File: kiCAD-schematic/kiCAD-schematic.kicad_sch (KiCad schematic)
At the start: 39 parts, among them J1 ext. power, J2 keyboard (usb-a), J3 keyboard (ps/2), Q1 2N222A, Q2 2N3904, Q3 2N3906, Q4 2N3904, SW1 ~RESET, SW2 POWER

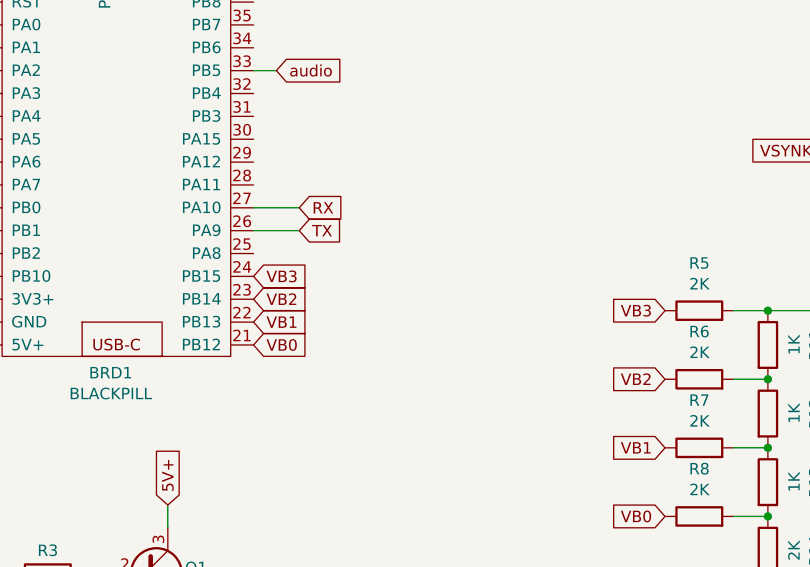
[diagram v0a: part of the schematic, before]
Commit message: modification de IF-SENSE
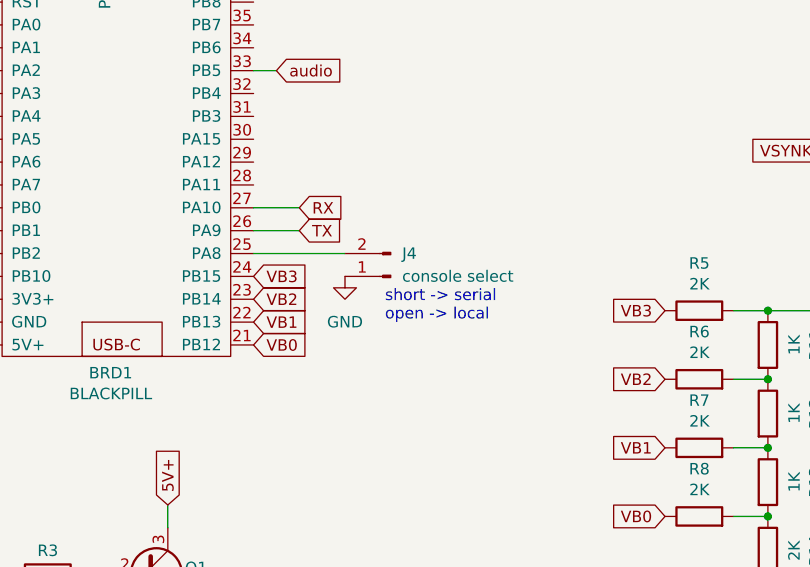
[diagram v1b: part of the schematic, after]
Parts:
- added J4: console select, symbol Connector:Conn_01x02_Male
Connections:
- net GND: now also J4.1 (Pin_1)
- net at BRD1.25 (PA8): now also J4.2 (Pin_2)
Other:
- note added: "short -> serial open -> local"
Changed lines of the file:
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@@
+    (stroke (width 0) (type default) (color 0 0 0 0))
+  )
+  (wire (pts (xy 163.83 110.49) (xy 173.99 110.49))
     (stroke (width 0) (type default) (color 0 0 0 0))
   )
@@
   (wire (pts (xy 210.82 16.51) (xy 214.63 16.51))
     (stroke (width 0) (type default) (color 0 0 0 0))
+  )
+  (text "short -> serial\nopen -> local" (at 178.435 118.11 0)
+    (effects (font (size 1.27 1.27)) (justify left bottom))
   )
   (text "keyboard connector\nalternative\n" (at 55.88 175.26 0)
@@
   (symbol (lib_id "power:GND") (at 214.63 35.56 0) (mirror y) (unit 1)
     (in_bom yes) (on_board yes)
-    (property "Reference" "#PWR011" (id 0) (at 214.63 41.91 0)
+    (property "Reference" "#PWR012" (id 0) (at 214.63 41.91 0)
       (effects (font (size 1.27 1.27)) hide)
     )
@@
   (symbol (lib_id "power:GND") (at 238.76 48.26 0) (unit 1)
     (in_bom yes) (on_board yes)
-    (property "Reference" "#PWR014" (id 0) (at 238.76 54.61 0)
+    (property "Reference" "#PWR015" (id 0) (at 238.76 54.61 0)
       (effects (font (size 1.27 1.27)) hide)
     )
@@
   (symbol (lib_id "power:GND") (at 248.92 133.35 0) (unit 1)
     (in_bom yes) (on_board yes)
-    (property "Reference" "#PWR015" (id 0) (at 248.92 139.7 0)
+    (property "Reference" "#PWR016" (id 0) (at 248.92 139.7 0)
       (effects (font (size 1.27 1.27)) hide)
     )
@@
   (symbol (lib_id "power:GND") (at 175.26 76.2 0) (unit 1)
     (in_bom yes) (on_board yes)
-    (property "Reference" "#PWR010" (id 0) (at 175.26 82.55 0)
+    (property "Reference" "#PWR011" (id 0) (at 175.26 82.55 0)
       (effects (font (size 1.27 1.27)) hide)
     )
@@
   (symbol (lib_id "power:GND") (at 234.95 133.35 0) (unit 1)
     (in_bom yes) (on_board yes)
-    (property "Reference" "#PWR013" (id 0) (at 234.95 139.7 0)
+    (property "Reference" "#PWR014" (id 0) (at 234.95 139.7 0)
       (effects (font (size 1.27 1.27)) hide)
     )
@@
   (symbol (lib_id "power:GND") (at 220.98 147.32 0) (unit 1)
     (in_bom yes) (on_board yes)
-    (property "Reference" "#PWR012" (id 0) (at 220.98 153.67 0)
+    (property "Reference" "#PWR013" (id 0) (at 220.98 153.67 0)
       (effects (font (size 1.27 1.27)) hide)
     )
@@
     (pin "2")
     (pin "3")
+  )
+  (symbol (lib_id "power:GND") (at 173.99 113.03 0) (unit 1)
+    (in_bom yes) (on_board yes) (fields_autoplaced)
+    (property "Reference" "#PWR010" (id 0) (at 173.99 119.38 0)
+      (effects (font (size 1.27 1.27)) hide)
+    )
+    (property "Value" "GND" (id 1) (at 173.99 118.11 0))
+    (property "Footprint" "" (id 2) (at 173.99 113.03 0)
+      (effects (font (size 1.27 1.27)) hide)
+    )
+    (property "Datasheet" "" (id 3) (at 173.99 113.03 0)
+      (effects (font (size 1.27 1.27)) hide)
+    )
+    (pin "1")
   )
   (symbol (lib_id "power:GND") (at 172.085 156.21 0) (unit 1)
@@
     (pin "2")
   )
+  (symbol (lib_id "Connector:Conn_01x02_Male") (at 179.07 113.03 180) (unit 1)
+    (in_bom yes) (on_board yes) (fields_autoplaced)
+    (property "Reference" "J4" (id 0) (at 180.34 110.4899 0)
+      (effects (font (size 1.27 1.27)) (justify right))
+    )
+    (property "Value" "console select" (id 1) (at 180.34 113.0299 0)
+      (effects (font (size 1.27 1.27)) (justify right))
+    )
+    (property "Footprint" "" (id 2) (at 179.07 113.03 0)
+      (effects (font (size 1.27 1.27)) hide)
+    )
+    (property "Datasheet" "~" (id 3) (at 179.07 113.03 0)
+      (effects (font (size 1.27 1.27)) hide)
+    )
+    (pin "1")
+    (pin "2")
+  )
   (sheet_instances
     (path "/" (page "1"))
@@
       (reference "#PWR09") (unit 1) (value "GND") (footprint "")
     )
+    (path "/293694f5-f84a-43cb-b18d-6048fb0e7311"
+      (reference "#PWR010") (unit 1) (value "GND") (footprint "")
+    )
     (path "/00000000-0000-0000-0000-00006002e243"
-      (reference "#PWR010") (unit 1) (value "GND") (footprint "")
+      (reference "#PWR011") (unit 1) (value "GND") (footprint "")
     )
     (path "/00000000-0000-0000-0000-00005ffbb8c6"
-      (reference "#PWR011") (unit 1) (value "GND") (footprint "")
+      (reference "#PWR012") (unit 1) (value "GND") (footprint "")
     )
     (path "/00000000-0000-0000-0000-0000606c01f2"
-      (reference "#PWR012") (unit 1) (value "GND") (footprint "")
+      (reference "#PWR013") (unit 1) (value "GND") (footprint "")
     )
     (path "/00000000-0000-0000-0000-0000606bce93"
-      (reference "#PWR013") (unit 1) (value "GND") (footprint "")
+      (reference "#PWR014") (unit 1) (value "GND") (footprint "")
     )
     (path "/00000000-0000-0000-0000-00005ffbd895"
-      (reference "#PWR014") (unit 1) (value "GND") (footprint "")
+      (reference "#PWR015") (unit 1) (value "GND") (footprint "")
     )
     (path "/00000000-0000-0000-0000-00005ffe2066"
-      (reference "#PWR015") (unit 1) (value "GND") (footprint "")
+      (reference "#PWR016") (unit 1) (value "GND") (footprint "")
     )
     (path "/00000000-0000-0000-0000-00005ffb52d6"
@@
       (reference "J3") (unit 1) (value "keyboard (ps/2)") (footprint "")
     )
+    (path "/e378ab9b-373b-45f1-b4f3-44620429fe99"
+      (reference "J4") (unit 1) (value "console select") (footprint "")
+    )
     (path "/a7b6ec0b-19e1-478b-92f2-5a0b45d45460"

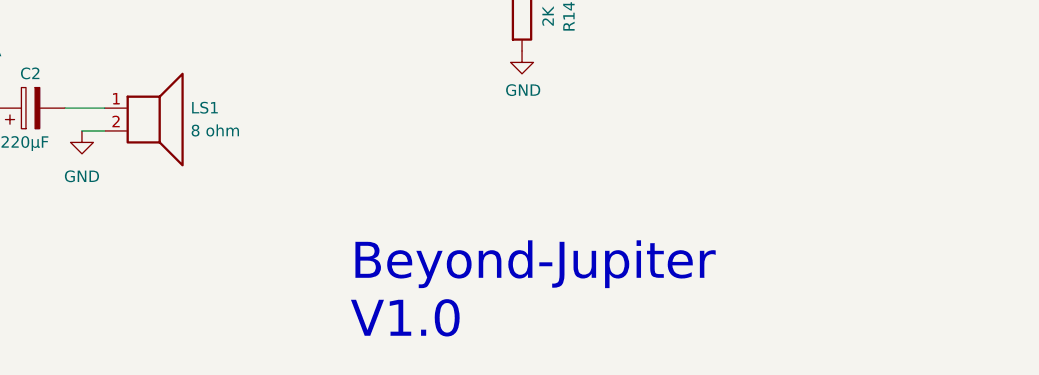
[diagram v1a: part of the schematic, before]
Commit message: mise à jour readme.md
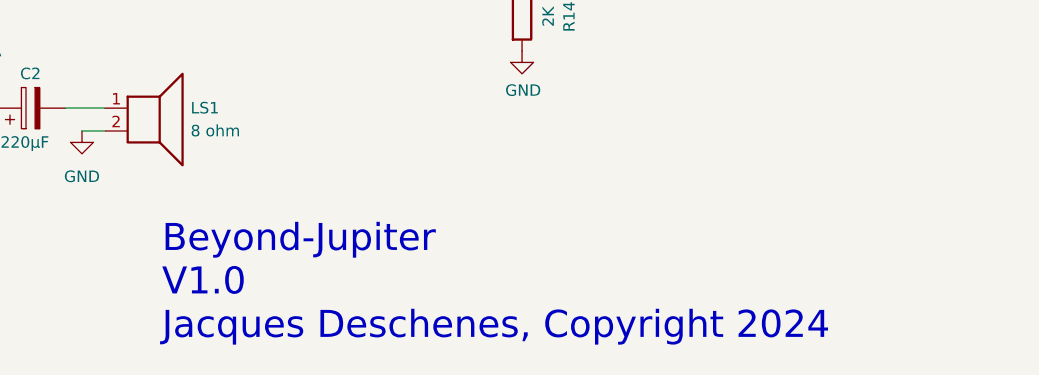
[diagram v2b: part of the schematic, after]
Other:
- note added: "Beyond-Jupiter V1.0 Jacques Deschenes, Copyright 2024"
- note removed: "Beyond-Jupiter V1.0"
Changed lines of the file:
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@@
     (effects (font (size 2.0066 2.0066)) (justify left bottom))
   )
-  (text "Beyond-Jupiter\nV1.0" (at 201.93 179.705 0)
-    (effects (font (size 4 4)) (justify left bottom))
+  (text "Beyond-Jupiter\nV1.0\nJacques Deschenes, Copyright 2024"
+    (at 180.975 179.705 0)
+    (effects (font (size 3 3)) (justify left bottom))
   )
   (text "PA4,PA5,PA6,PA7\nUSED BY W25Q128\nON board SPI FLASH"
